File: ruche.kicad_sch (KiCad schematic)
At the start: 46 parts, among them IC2 MAX17048G+, IC3 L86-M33, IC4 SHT41-AD1B-R3, J13 Micro_SD_Card, J19 Conn_01x02, U2 MS5611-01BA, U3 XC6220B331MR, U5 XC6220B331MR, U8 E32-868T20D, U9 XC6220B331MR

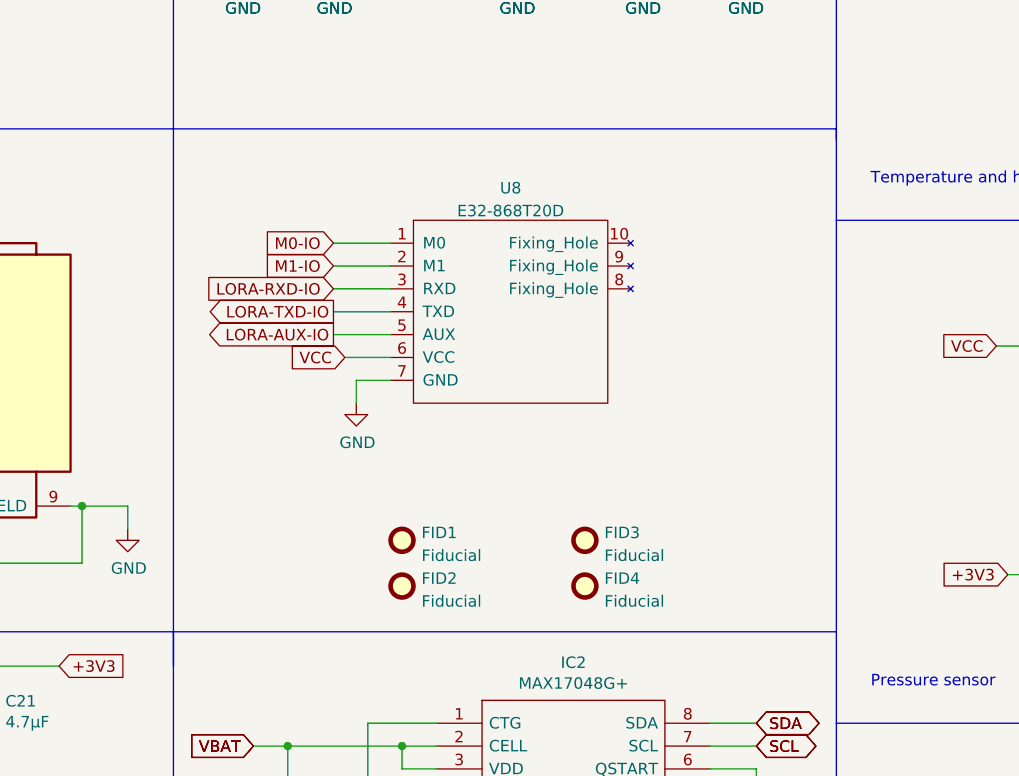
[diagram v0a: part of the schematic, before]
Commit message: update
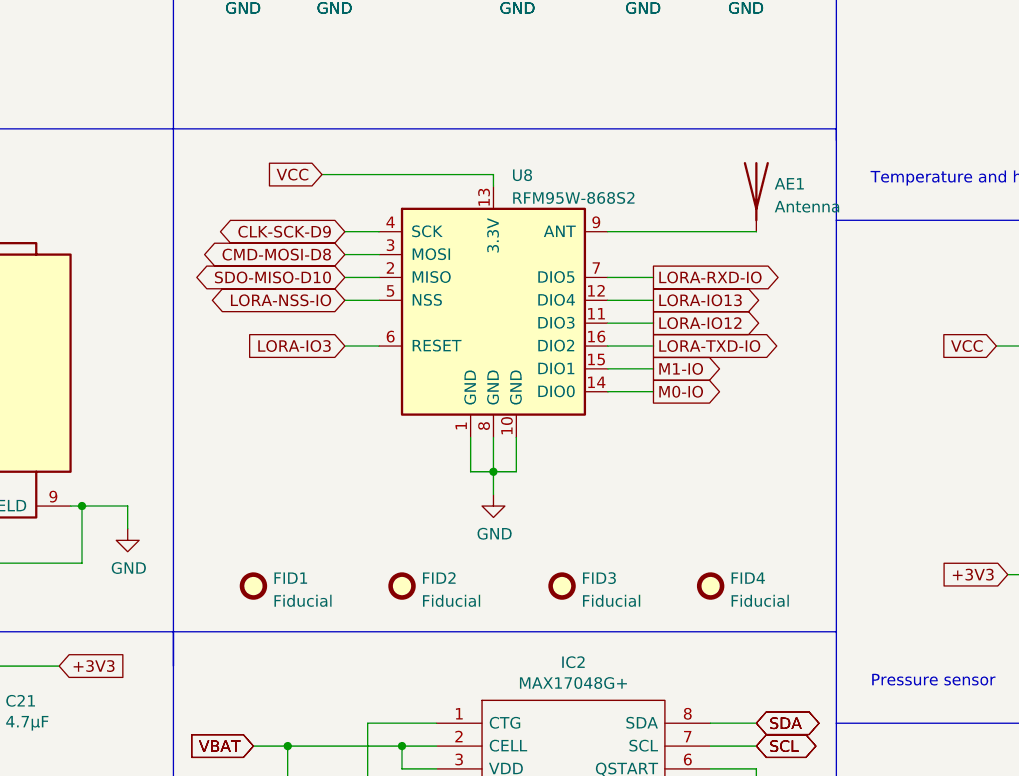
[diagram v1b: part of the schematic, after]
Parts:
- removed U8: E32-868T20D, Empreintes:Ebyte, symbol E32-xxxT20D:E32-868T20D
- added AE1: Antenna, Connector_Coaxial:U.FL_Hirose_U.FL-R-SMT-1_Vertical, symbol Device:Antenna
- added U8: RFM95W-868S2, RF_Module:HOPERF_RFM9XW_SMD, symbol RF_Module:RFM95W-868S2
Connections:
- net CLK-SCK-D9: now also U8.4 (SCK)
- net CMD-MOSI-D8: now also U8.3 (MOSI)
- net GND: now also U8.1 (GND), U8.10 (GND), U8.8 (GND)
- net LORA-RXD-IO: now also U8.7 (DIO5)
- net LORA-TXD-IO: now also U8.16 (DIO2)
- net M0-IO: now also U8.14 (DIO0)
- net M1-IO: now also U8.15 (DIO1)
- net SDO-MISO-D10: now also U8.2 (MISO)
- net VCC: now also U8.13 (3.3V)
- new net: AE1.1 (A), U8.9 (ANT)
- new net LORA-IO12: U8.11 (DIO3)
- new net LORA-IO13: U8.12 (DIO4)
- new net LORA-IO3: U8.6 (RESET)
- new net LORA-NSS-IO: U8.5 (NSS)
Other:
- moved on the sheet: FID1, FID3, FID4

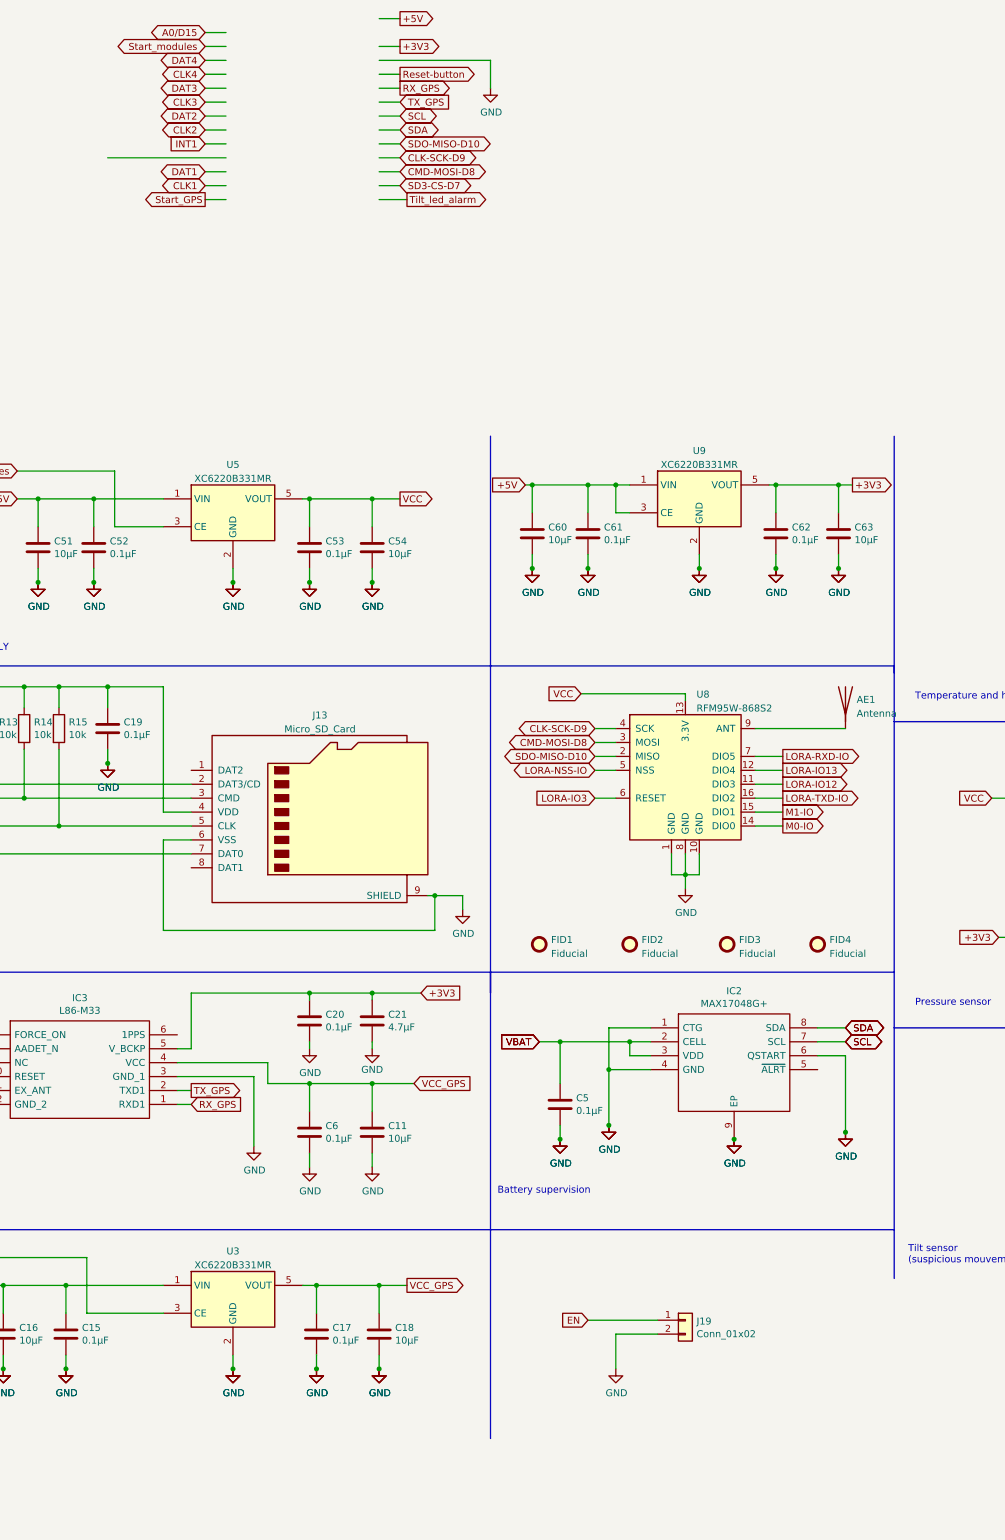
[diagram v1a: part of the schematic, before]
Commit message: update
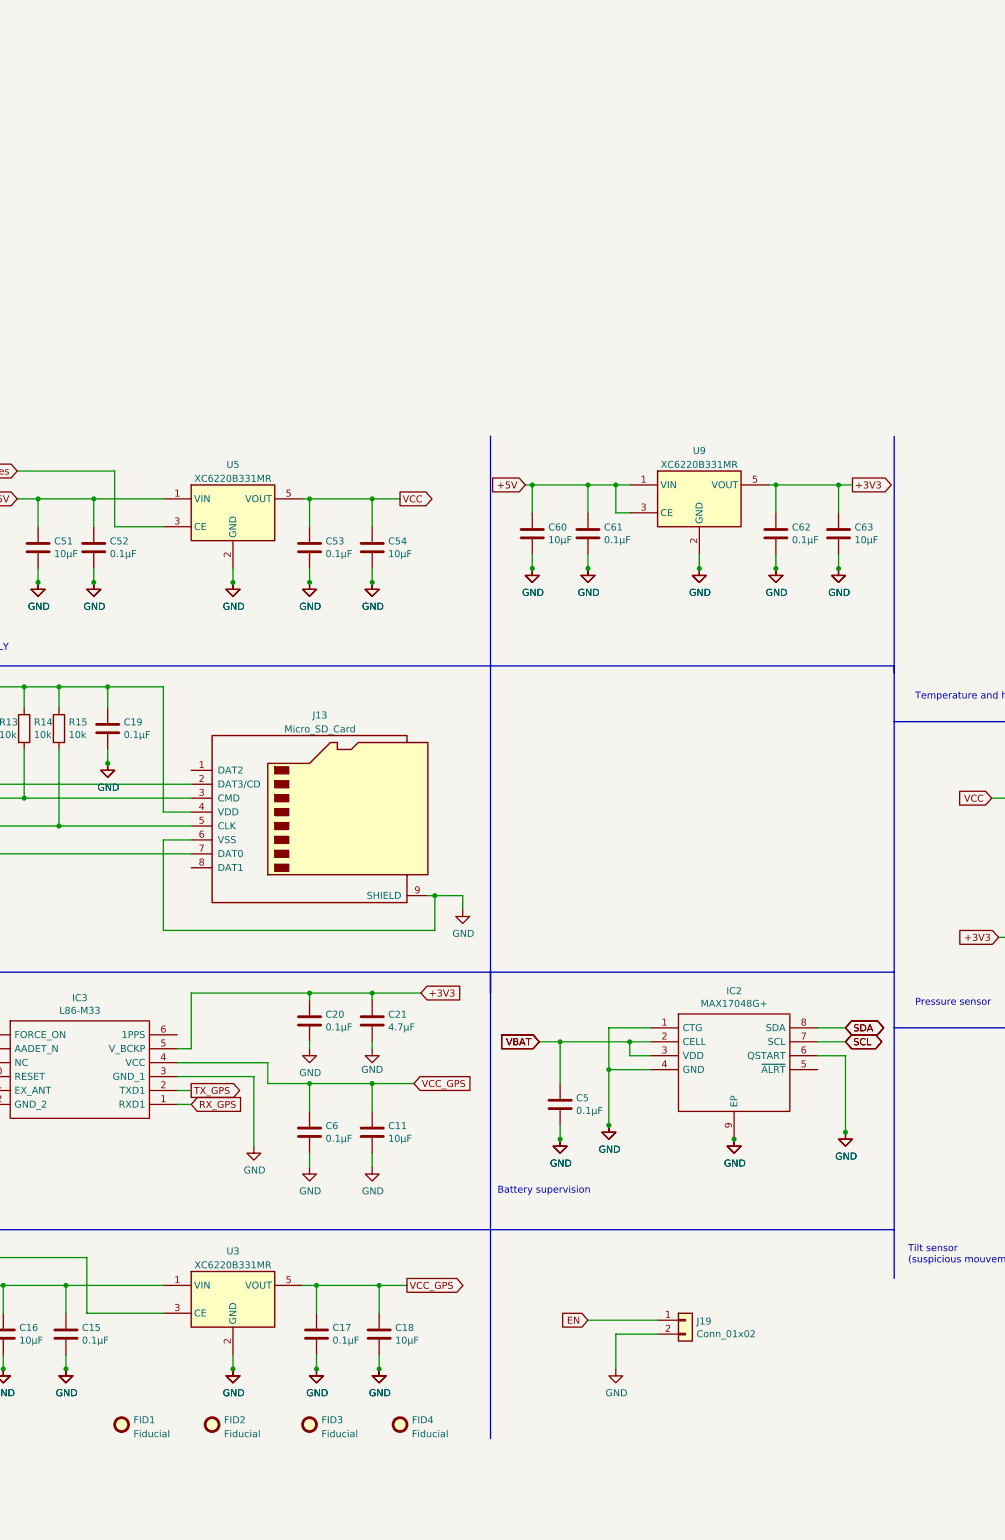
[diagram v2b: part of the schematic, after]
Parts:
- removed AE1: Antenna, Connector_Coaxial:U.FL_Hirose_U.FL-R-SMT-1_Vertical, symbol Device:Antenna
- removed U8: RFM95W-868S2, RF_Module:HOPERF_RFM9XW_SMD, symbol RF_Module:RFM95W-868S2
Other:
- moved on the sheet: FID1, FID2, FID3, FID4
